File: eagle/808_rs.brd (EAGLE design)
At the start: 100 x 80 mm, 75 parts, among them IC1 TL072P, IC2 TL072P, Q1 2SK30, Q59 2N3904, Q60 2N3906, Q61 2N3904, Q62 2N3904, Q63 2N3904, SW8 808_LT_MSS42_SW_4PDT

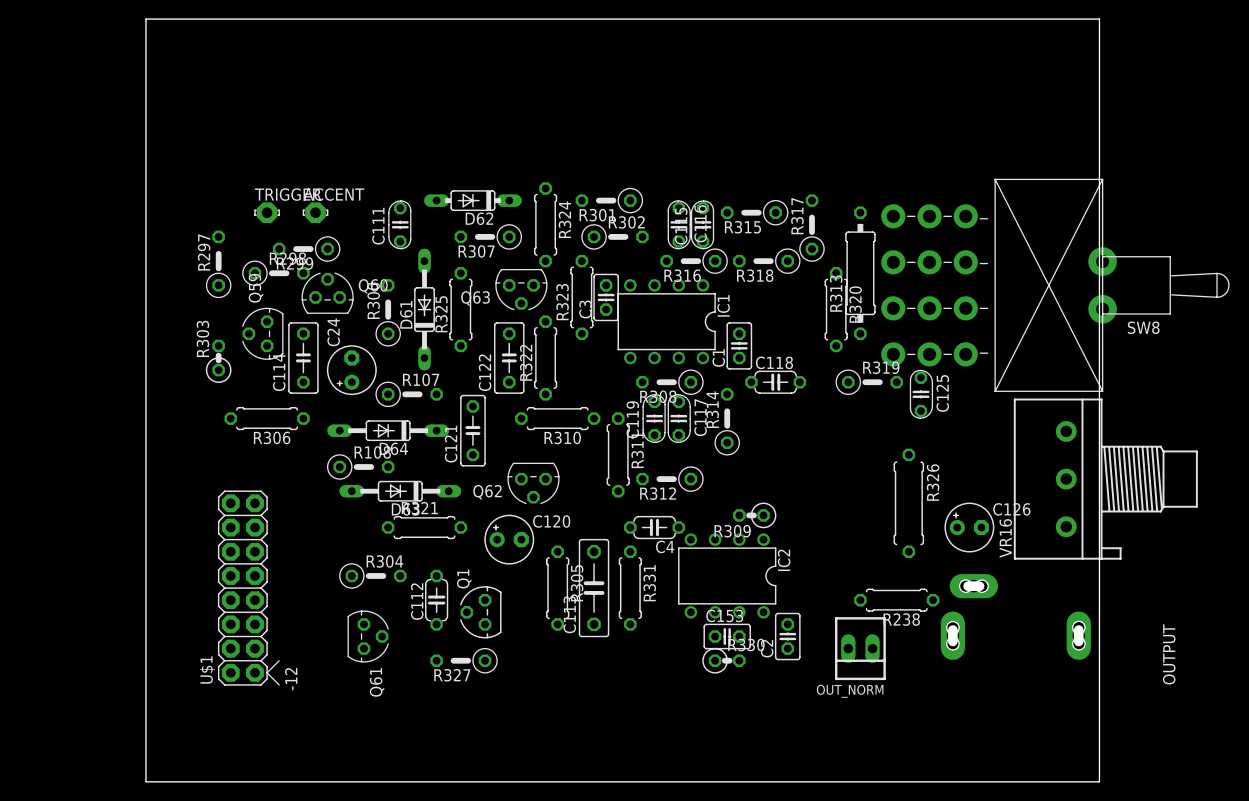
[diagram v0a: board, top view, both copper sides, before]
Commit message: routed
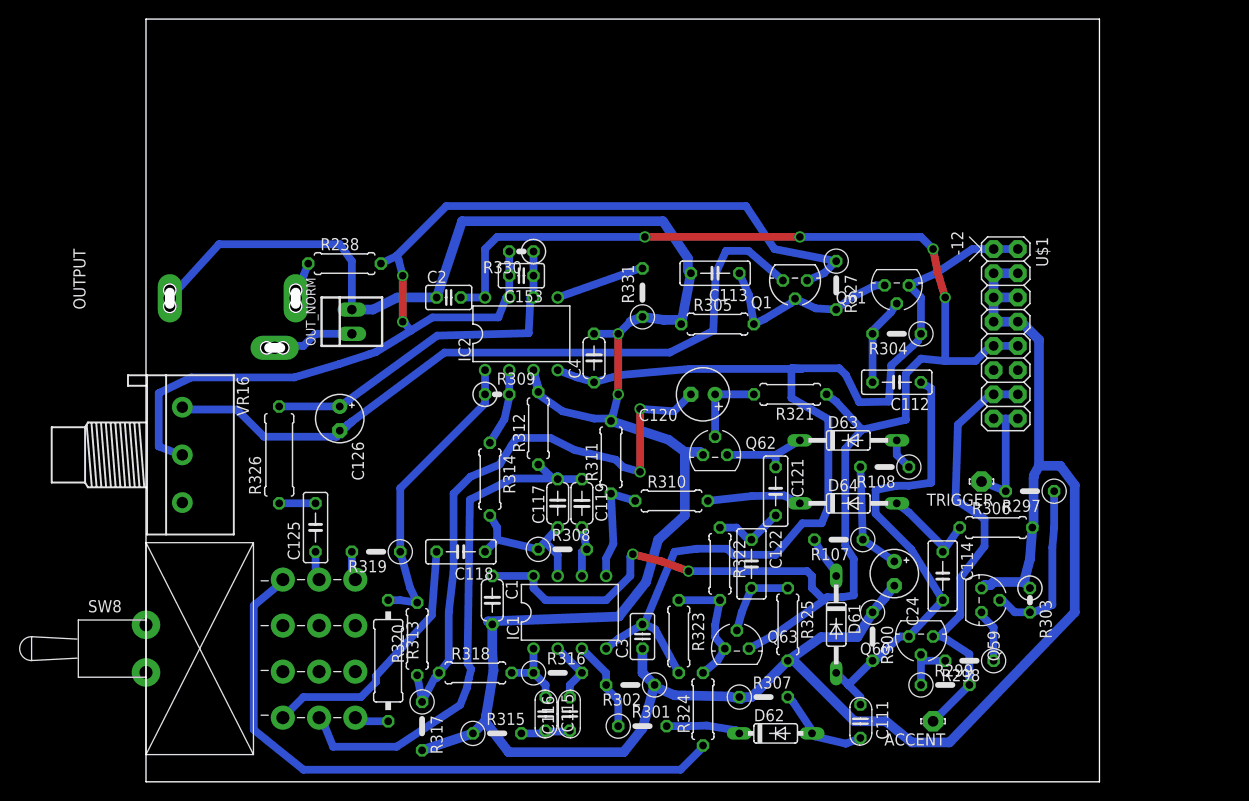
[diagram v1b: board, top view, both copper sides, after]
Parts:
- C1: device TR808clone:C025-025X050 -> TR808clone:C050-024X044
- C112, C118: device TR808clone:C050-024X044 -> TR808clone:C050-025X075
- C113: device TR808clone:C075-032X103 -> TR808clone:C050-025X075
- C117, C119: device TR808clone:C035-025X75 -> TR808clone:C050-024X044
- C120: device TR808clone:E2,5-5 -> TR808clone:E2,5-6
- C125: device TR808clone:C035-025X75 -> TR808clone:C050-025X075
- R312, R314, R318: device TR808clone:0207/5V -> TR808clone:0207/7
- R331: device TR808clone:0207/7 -> TR808clone:0207/5V
- moved SW8 107.3 mm to (0.00, 14.0), turned to 270 degrees
- moved OUTPUT 103.5 mm to (0.00, 45.7), turned to 90 degrees
- moved VR16 92.7 mm to (3.81, 34.3), turned to 270 degrees
- moved R303 88.8 mm to (92.7, 19.1), turned to 270 degrees
- moved R297 88.4 mm to (92.7, 30.5), turned to 180 degrees
- moved U$1 86.1 mm to (90.2, 49.5), turned to 270 degrees
- moved ACCENT 83.9 mm to (82.5, 6.35), turned to 180 degrees
- moved R298 83.0 mm to (86.4, 12.7), turned to 180 degrees
- moved R299 81.4 mm to (83.8, 10.2), turned to 0 degrees
- moved TRIGGER 80.1 mm to (87.6, 31.5), turned to 180 degrees
- moved Q59 80.0 mm to (87.6, 19.1), turned to 270 degrees
- moved R306 77.3 mm to (89.2, 26.7), turned to 0 degrees
- moved Q60 71.7 mm to (81.3, 15.2), turned to 180 degrees
- moved C111 71.0 mm to (74.9, 6.35), turned to 270 degrees
- moved C114 70.8 mm to (83.6, 21.6), turned to 270 degrees
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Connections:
- net N$2: now also C125.1; no longer C125.P$1
- net N$338: now also C117.2, C119.1; no longer C117.P$2, C119.P$1
- net N$339: now also C119.2; no longer C119.P$2
- net N$340: now also C117.1; no longer C117.P$1
- net N$347: now also C125.2; no longer C125.P$2
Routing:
- net GND: track 0.00 -> 336.7 mm, vias 0 -> 2
- net +12V: track 0.00 -> 168.5 mm, vias 0 -> 6
- net -12V: track 0.00 -> 121.3 mm
- net N$8: track 0.00 -> 117.8 mm, vias 0 -> 2
- net N$351: track 0.00 -> 79.6 mm
- net N$6: track 0.00 -> 67.2 mm
- net N$355: track 0.00 -> 61.3 mm, vias 0 -> 2
- net N$338: track 0.00 -> 54.7 mm
- net N$357: track 0.00 -> 49.2 mm
- net TRIG: track 0.00 -> 46.0 mm
- net N$348: track 0.00 -> 37.5 mm
- net N$344: track 0.00 -> 31.4 mm
- net N$165: track 0.00 -> 27.3 mm
- net N$161: track 0.00 -> 21.1 mm
- net N$318: track 0.00 -> 18.1 mm
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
